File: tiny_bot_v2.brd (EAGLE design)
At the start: 48.3 x 80.8 mm, 31 parts, among them IC1 SN754410PDIP, U1 ATMEGA328P_PDIP, X1 16 MHz

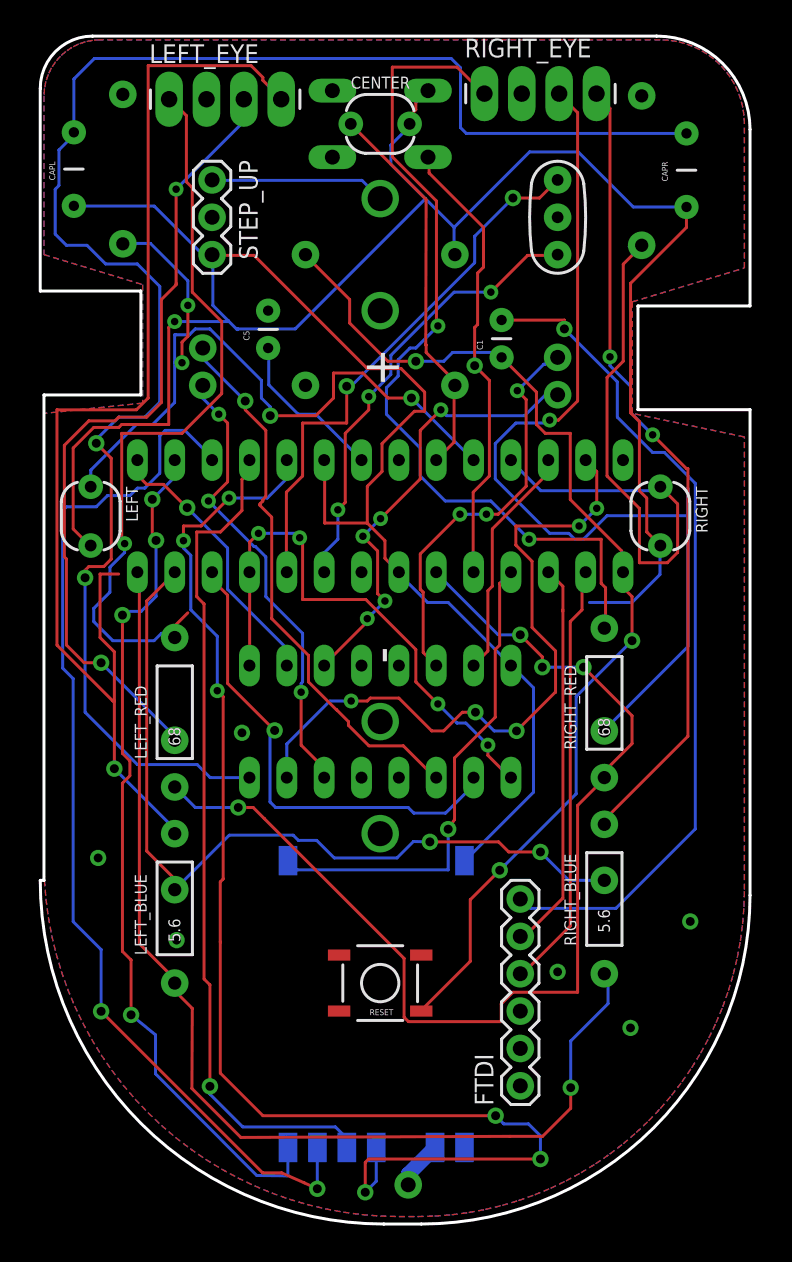
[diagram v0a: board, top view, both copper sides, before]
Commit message: Adding gerbers
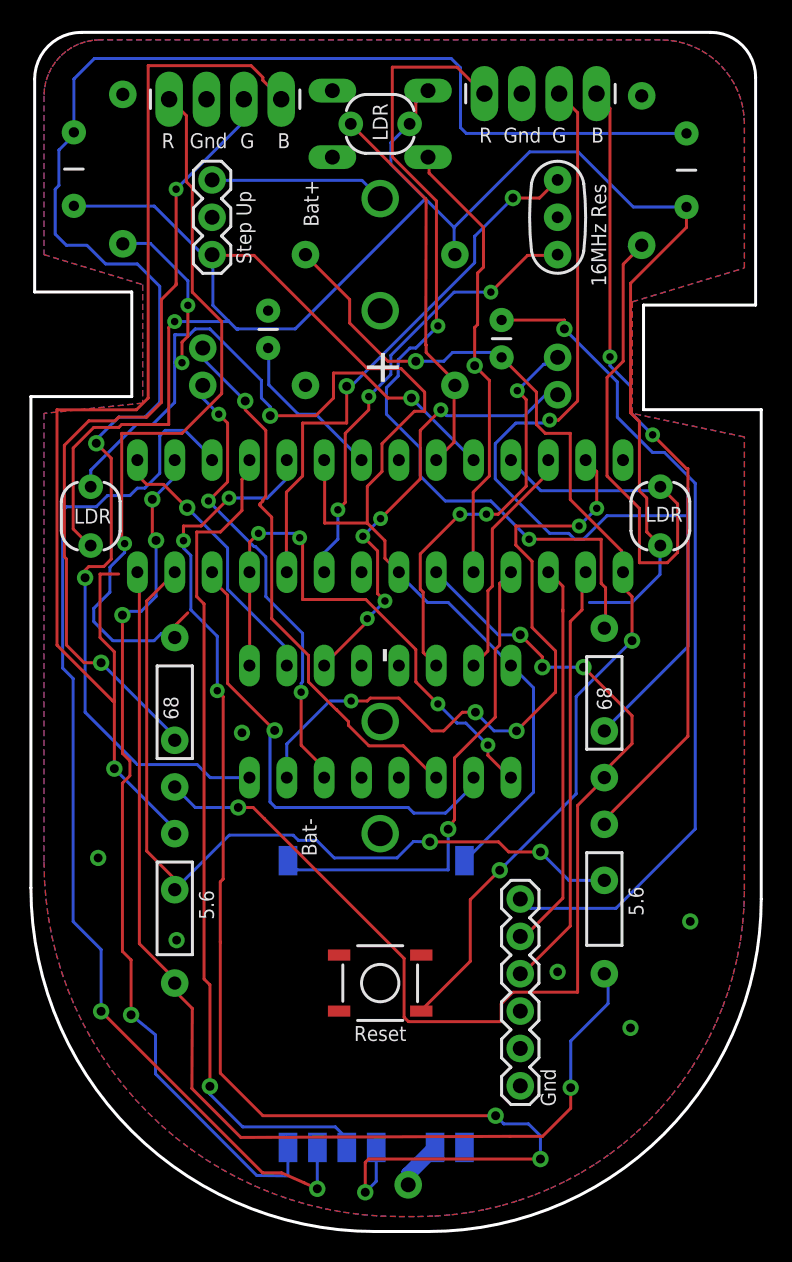
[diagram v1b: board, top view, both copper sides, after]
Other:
- board size 48.3 x 80.8 mm -> 49.7 x 81.5 mm
- board text added: "16MHz Res"
- board text added: "ATMEGA328"
- board text added: "Ant"
- board text added: "B"
- board text added: "Bat+"
- board text added: "Bat-"
- board text added: "G"
- board text added: "Gnd"
- board text added: "LDR"
- board text added: "Left Motor"
- board text added: "Motor Driver"
- board text added: "Nose"
- board text added: "R"
- board text added: "RFM69W"
- board text added: "Reset"
- board text added: "Right Motor"
- board text added: "Step Up"
